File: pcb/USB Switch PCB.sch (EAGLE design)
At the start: 16 parts, among them Q1 2N7002P, Q2 2N7002P, U1 D1MINI, X1 UE27-USBA, X2 HLP511-USBMICROB

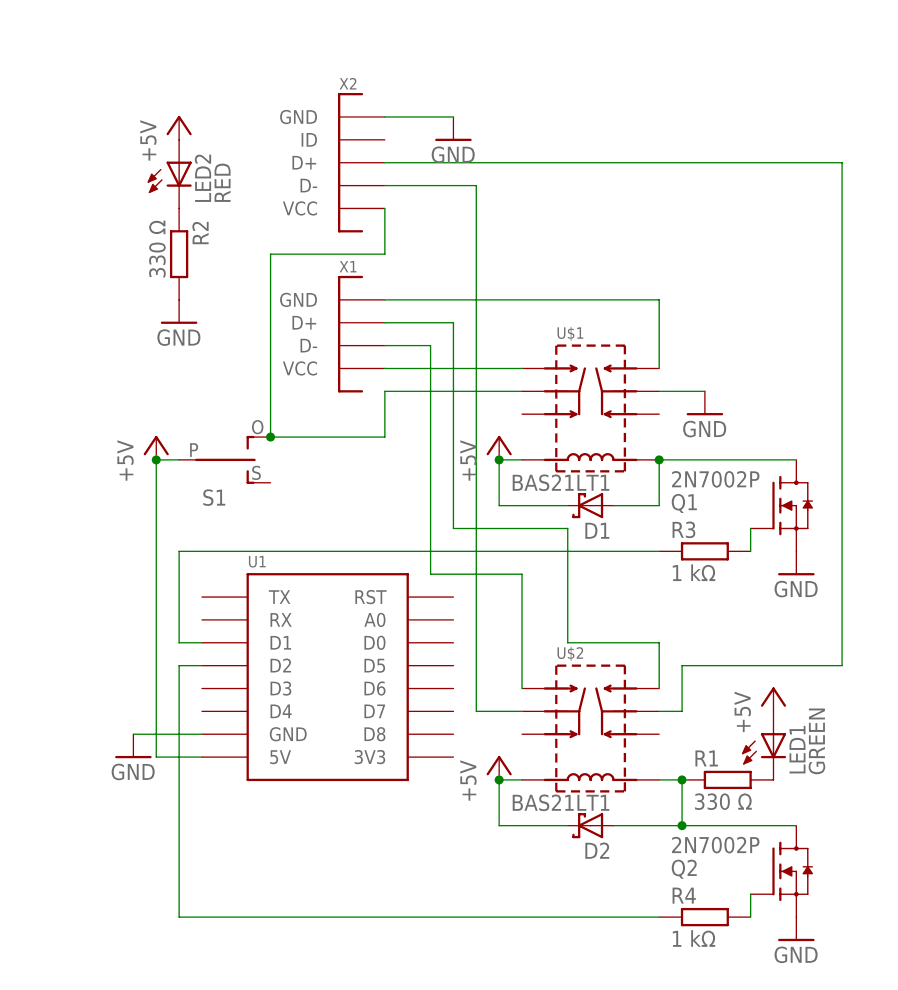
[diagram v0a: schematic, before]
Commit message: More work!
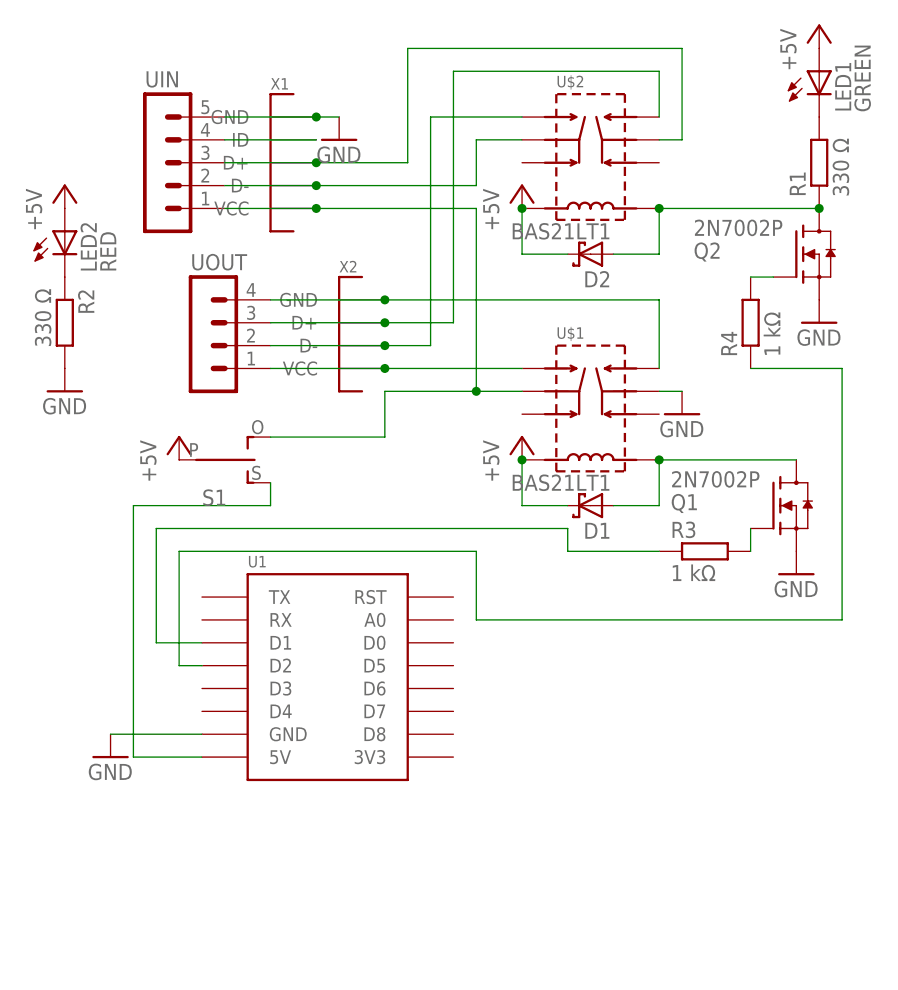
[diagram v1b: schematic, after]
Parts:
- added UIN: (no value), con-lstb:MA05-1
- added UOUT: (no value), con-lstb:MA04-1
- X1: value UE27-USBA -> AMPHENOL-0001LF; device USB Switch PCB:UE27-USBA -> USB Switch PCB:AMPHENOL-0001LF
- X2: value HLP511-USBMICROB -> UE27-USBA; device USB Switch PCB:HLP511-USBMICROB -> USB Switch PCB:UE27-USBA
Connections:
- net N$5 renamed PWRON
- net N$7 renamed DATAON
- removed net N$10: U$1.A2, X1.GND
- removed net N$11: U$2.A1, X1.D-
- removed net N$12: U$2.A2, X1.D+
- removed net N$13: S1.O, U$1.C1, X2.VCC
- removed net N$14: U$2.C2, X2.D+
- removed net N$15: U$2.C1, X2.D-
- removed net N$9: U$1.A1, X1.VCC
- new net 5VESP: S1.S, U1.5V
- new net 5VUSB: S1.O, U$1.C1, UIN.1, X1.VCC
- new net D+: U$2.C2, UIN.3, X1.D+
- new net D+O: U$2.A2, UOUT.3, X2.D+
- new net D-: U$2.C1, UIN.2, X1.D-
- new net D-O: U$2.A1, UOUT.2, X2.D-
- new net GNDO: U$1.A2, UOUT.4, X2.GND
- new net N$16: UIN.4, X1.ID
- new net VCC0: U$1.A1, UOUT.1, X2.VCC
- net +5V: no longer U1.5V
- net GND: now also UIN.5, X1.GND; no longer X2.GND
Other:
- moved on the sheet: D2, LED1, LED2, Q2, R1, R2, R4, U$2
